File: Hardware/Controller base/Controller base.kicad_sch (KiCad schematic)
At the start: 37 parts, among them J1 USB_C_Receptacle_USB2.0_16P, J2 Conn_01x05_Pin, J3 right face mod, J4 left face mod, J5 left sholder, J6 right sholder, SW1 SW_Push, SW2 SW_Push, SW3 SW_Push, SW4 SW_Push, U1 AZ1117CH-3.3TRG1, U2 ESP32-S3-WROOM-1U-N4

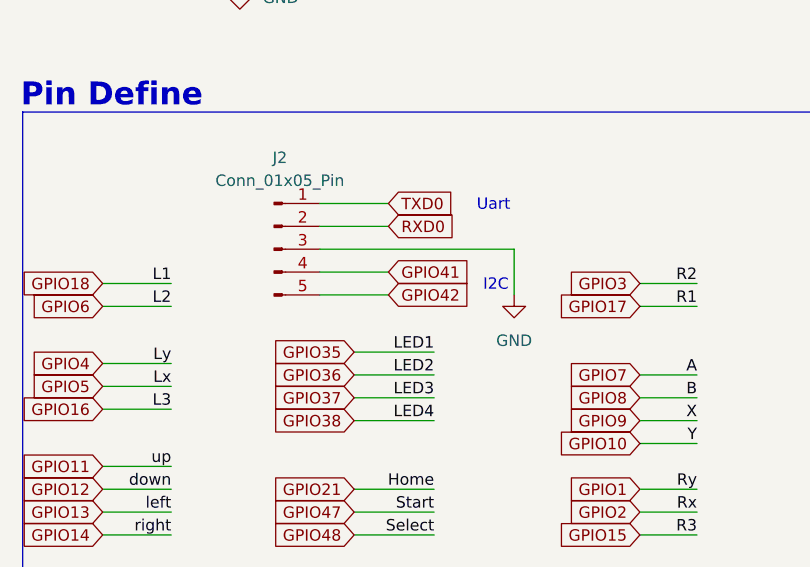
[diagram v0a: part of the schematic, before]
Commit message: update
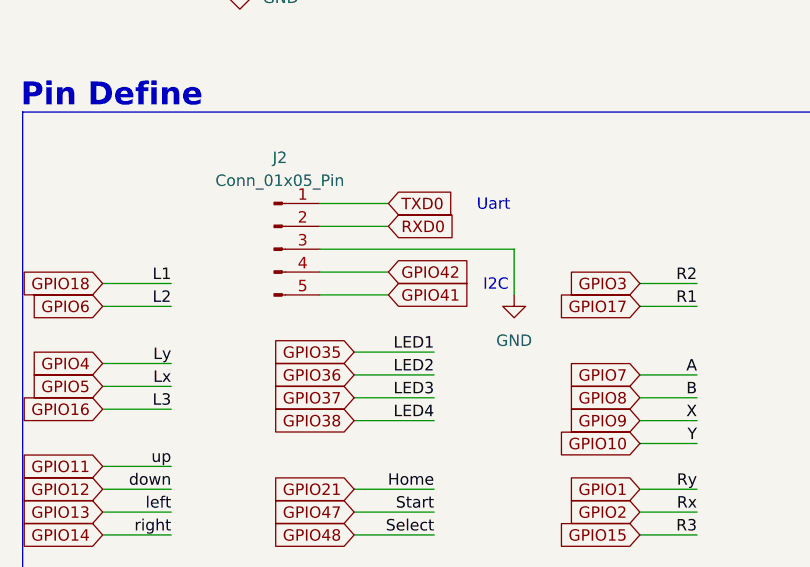
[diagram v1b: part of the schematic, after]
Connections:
- net GPIO41: now also J2.5 (Pin_5); no longer J2.4 (Pin_4)
- net GPIO42: now also J2.4 (Pin_4); no longer J2.5 (Pin_5)
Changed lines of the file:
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@@
 	(wire
 		(pts
-			(xy 176.53 139.7) (xy 179.07 139.7)
+			(xy 53.34 162.56) (xy 45.72 162.56)
 		)
 		(stroke
@@
 	(wire
 		(pts
-			(xy 21.59 189.23) (xy 29.21 189.23)
+			(xy 176.53 139.7) (xy 179.07 139.7)
 		)
 		(stroke
@@
 	(wire
 		(pts
-			(xy 115.57 44.45) (xy 109.22 44.45)
+			(xy 21.59 189.23) (xy 29.21 189.23)
 		)
 		(stroke
@@
 	(wire
 		(pts
-			(xy 45.72 162.56) (xy 53.34 162.56)
+			(xy 115.57 44.45) (xy 109.22 44.45)
 		)
 		(stroke
@@
 	(wire
 		(pts
-			(xy 45.72 165.1) (xy 53.34 165.1)
+			(xy 152.4 27.94) (xy 152.4 31.75)
 		)
 		(stroke
@@
 	(wire
 		(pts
-			(xy 152.4 27.94) (xy 152.4 31.75)
+			(xy 255.27 153.67) (xy 255.27 154.94)
 		)
 		(stroke
@@
 	(wire
 		(pts
-			(xy 255.27 153.67) (xy 255.27 154.94)
+			(xy 38.1 80.01) (xy 41.91 80.01)
 		)
 		(stroke
@@
 	(wire
 		(pts
-			(xy 38.1 80.01) (xy 41.91 80.01)
+			(xy 53.34 165.1) (xy 45.72 165.1)
 		)
 		(stroke
@@
 	(global_label "GPIO41"
 		(shape input)
-		(at 53.34 162.56 0)
+		(at 53.34 165.1 0)
 		(fields_autoplaced yes)
 		(effects
@@
 		)
 		(property "Intersheetrefs" "${INTERSHEET_REFS}"
-			(at 63.2195 162.56 0)
+			(at 63.2195 165.1 0)
 			(effects
 				(font
@@
 	(global_label "GPIO42"
 		(shape input)
-		(at 53.34 165.1 0)
+		(at 53.34 162.56 0)
 		(fields_autoplaced yes)
 		(effects
@@
 		)
 		(property "Intersheetrefs" "${INTERSHEET_REFS}"
-			(at 63.2195 165.1 0)
+			(at 63.2195 162.56 0)
 			(effects
 				(font

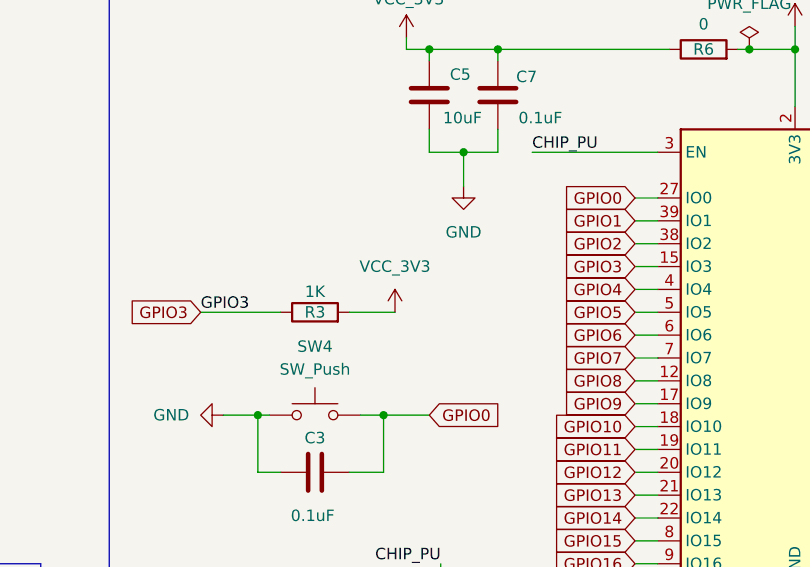
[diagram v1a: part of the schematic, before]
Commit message: update pcb
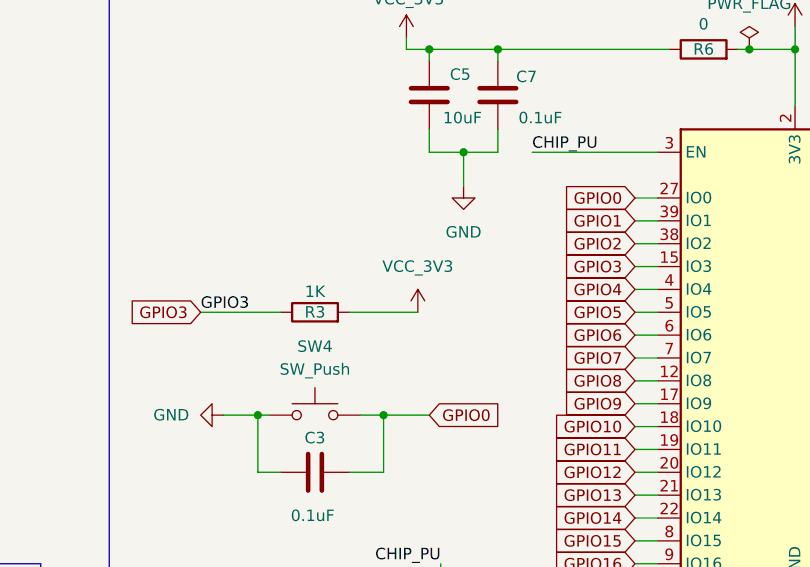
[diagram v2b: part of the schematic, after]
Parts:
- C3: footprint Capacitor_SMD:C_0805_2012Metric_Pad1.18x1.45mm_HandSolder -> Capacitor_SMD:C_0603_1608Metric_Pad1.08x0.95mm_HandSolder
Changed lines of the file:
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@@
 	(wire
 		(pts
-			(xy 144.78 116.84) (xy 149.86 116.84)
+			(xy 144.78 116.84) (xy 152.4 116.84)
 		)
 		(stroke
@@
 	(symbol
 		(lib_id "Library:+3V3")
-		(at 149.86 116.84 0)
+		(at 152.4 116.84 0)
 		(unit 1)
 		(exclude_from_sim no)
@@
 		(fields_autoplaced yes)
 		(property "Reference" "#PWR011"
-			(at 149.86 120.65 0)
+			(at 152.4 120.65 0)
 			(effects
 				(font
@@
 		)
 		(property "Value" "VCC_3V3"
-			(at 149.86 111.76 0)
+			(at 152.4 111.76 0)
 			(effects
 				(font
@@
 		)
 		(property "Footprint" ""
-			(at 149.86 116.84 0)
+			(at 152.4 116.84 0)
 			(effects
 				(font
@@
 		)
 		(property "Datasheet" ""
-			(at 149.86 116.84 0)
+			(at 152.4 116.84 0)
 			(effects
 				(font
@@
 		)
 		(property "Description" "Power symbol creates a global label with name \"+3V3\""
-			(at 149.86 116.84 0)
+			(at 152.4 116.84 0)
 			(effects
 				(font
@@
 			)
 		)
-		(property "Footprint" "Capacitor_SMD:C_0805_2012Metric_Pad1.18x1.45mm_HandSolder"
+		(property "Footprint" "Capacitor_SMD:C_0603_1608Metric_Pad1.08x0.95mm_HandSolder"
 			(at 144.78 133.6548 0)
 			(effects
